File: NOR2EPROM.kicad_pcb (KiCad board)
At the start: 2 copper layers, 9 parts, among them U1 SN74LVC245, U2 SN74LVC245, U3 MX29LV320, U4 27C322, U5 SN74LVC245, U6 SN74HCT245, U7 SN74HCT245, U8 LD1117S33TR_SOT223

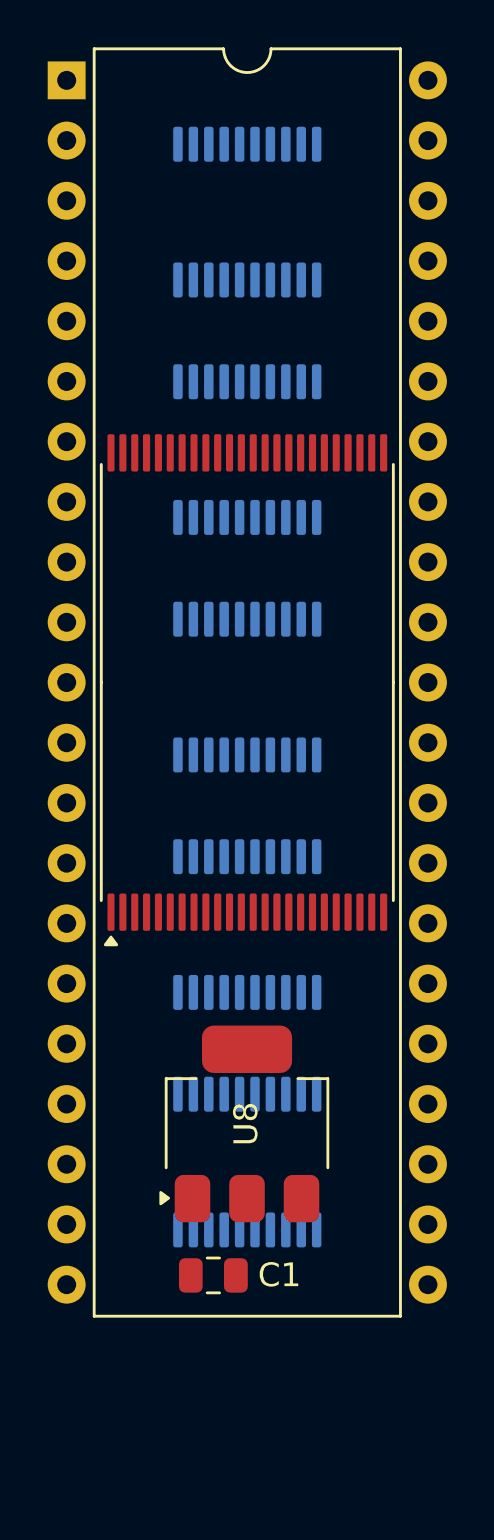
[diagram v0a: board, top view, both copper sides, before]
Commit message: routing checkpoint
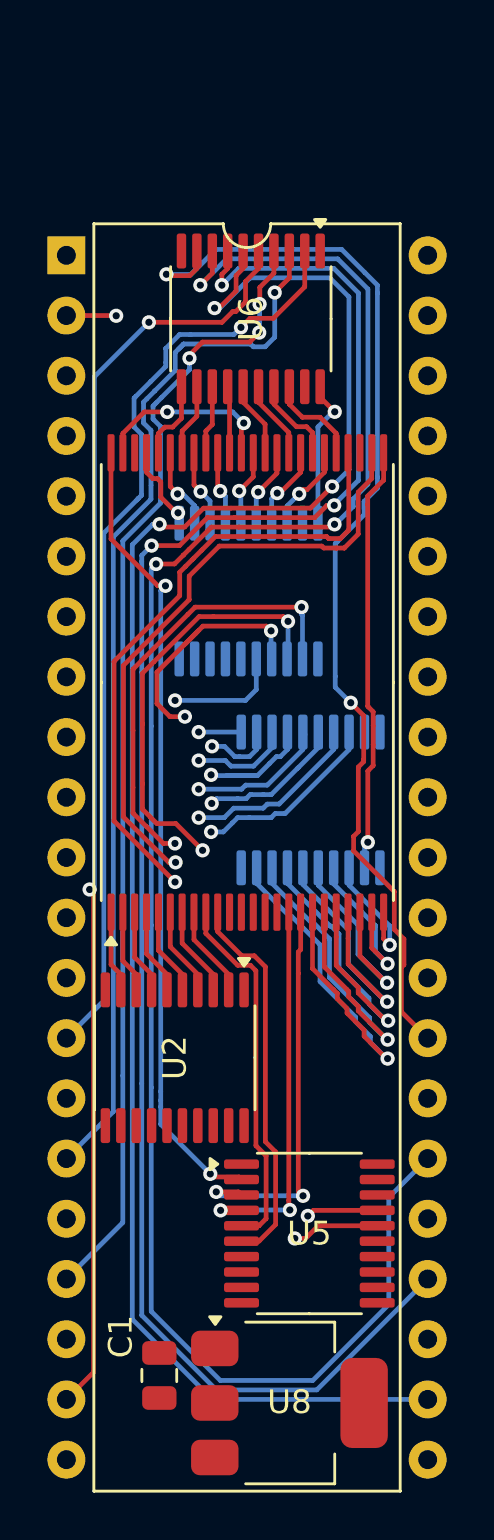
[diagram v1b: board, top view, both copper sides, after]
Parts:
- U2, U5, U6: moved to F.Cu
- moved U2 25.8 mm to (112.4, 103.5), turned to -90 degrees
- moved U6 25.6 mm to (115.6, 72.3), turned to -90 degrees
- moved U1 24.9 mm to (118.1, 92.6)
- moved U7 24.1 mm to (115.5, 83.8)
- moved U5 23.2 mm to (118.1, 110.9), turned to 0 degrees
- moved U8 11.9 mm to (117.2, 118.1), turned to 0 degrees
- moved U4 7.38 mm to (107.8, 69.7)
- moved C1 4.80 mm to (111.8, 116.9), turned to 90 degrees
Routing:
- net EPROM_Q6: track 0.00 -> 79.5 mm, vias 0 -> 3
- net EPROM_Q4: track 0.00 -> 73.9 mm, vias 0 -> 3
- net EPROM_Q5: track 0.00 -> 73.8 mm, vias 0 -> 3
- net EPROM_Q3: track 0.00 -> 53.9 mm, vias 0 -> 2
- net EPROM_A18: track 0.00 -> 49.5 mm, vias 0 -> 1
- net EPROM_Q2: track 0.00 -> 48.5 mm, vias 0 -> 3
- net EPROM_A17: track 0.00 -> 47.7 mm, vias 0 -> 2
- net EPROM_Q7: track 0.00 -> 47.1 mm, vias 0 -> 2
- net EPROM_Q1: track 0.00 -> 45.1 mm, vias 0 -> 1
- net EPROM_Q11: track 0.00 -> 41.6 mm, vias 0 -> 1
- net EPROM_Q10: track 0.00 -> 40.7 mm, vias 0 -> 2
- net EPROM_Q0: track 0.00 -> 39.8 mm, vias 0 -> 1
- net EPROM_Q9: track 0.00 -> 35.7 mm, vias 0 -> 2
- net NOR_A16: track 0.00 -> 33.9 mm, vias 0 -> 2
- net OUTPUT_ENABLE: track 0.00 -> 32.8 mm, vias 0 -> 1
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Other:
- copper layers 2 -> 4
